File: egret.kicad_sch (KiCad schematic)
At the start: 36 parts, among them J6 ADB, Q1 MMBT3904, U10 EGRET, U12 LS1126, Y1 S3238E

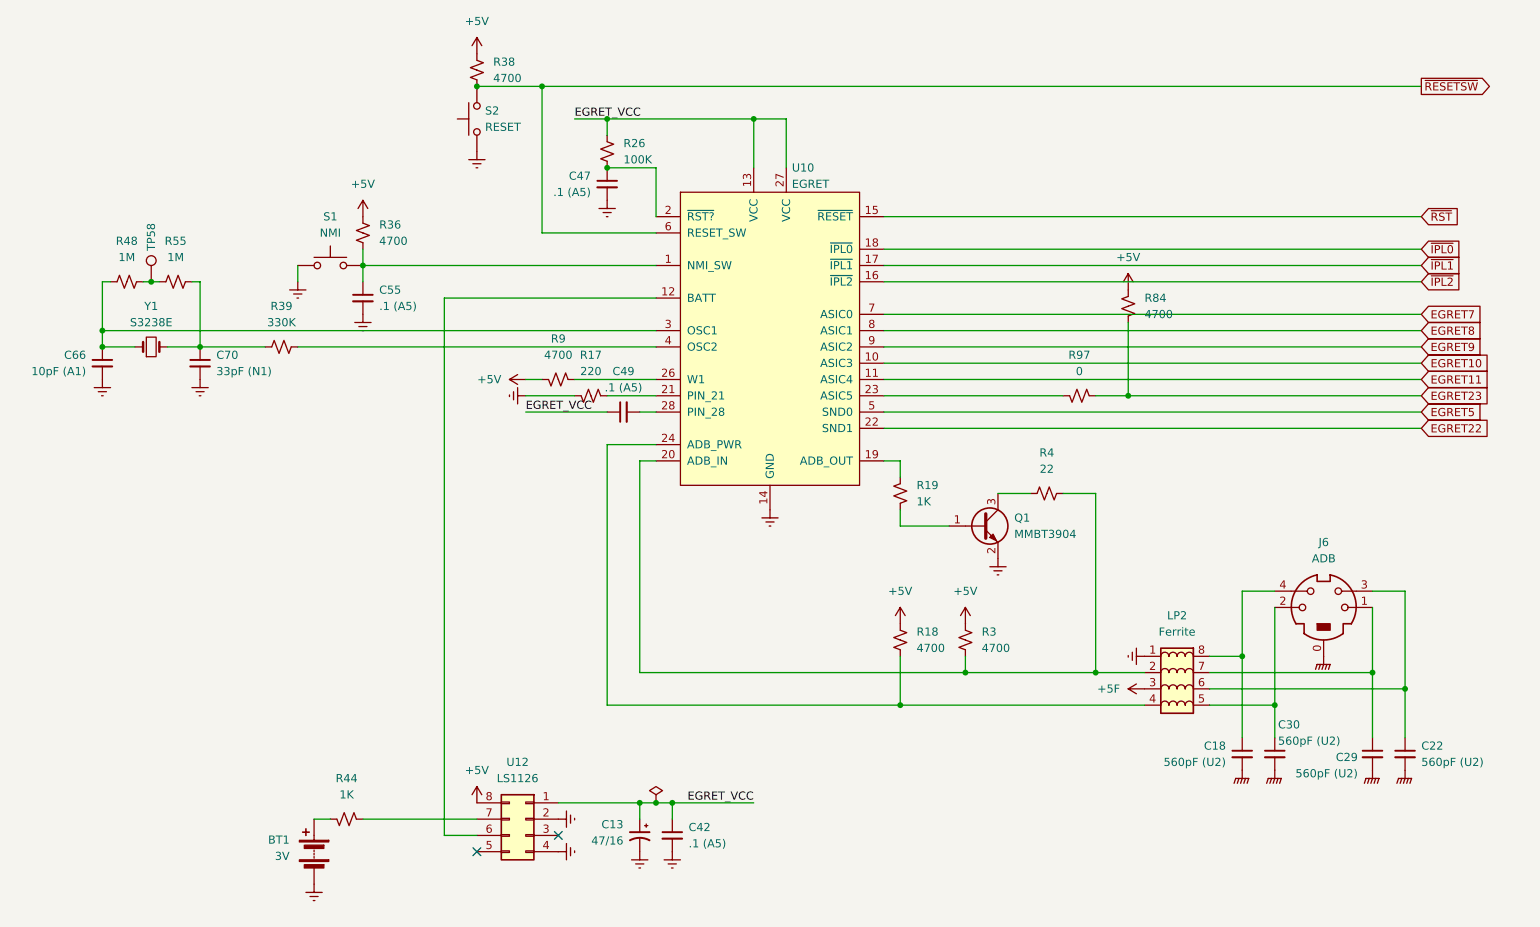
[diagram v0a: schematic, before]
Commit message: More schematic cleanup
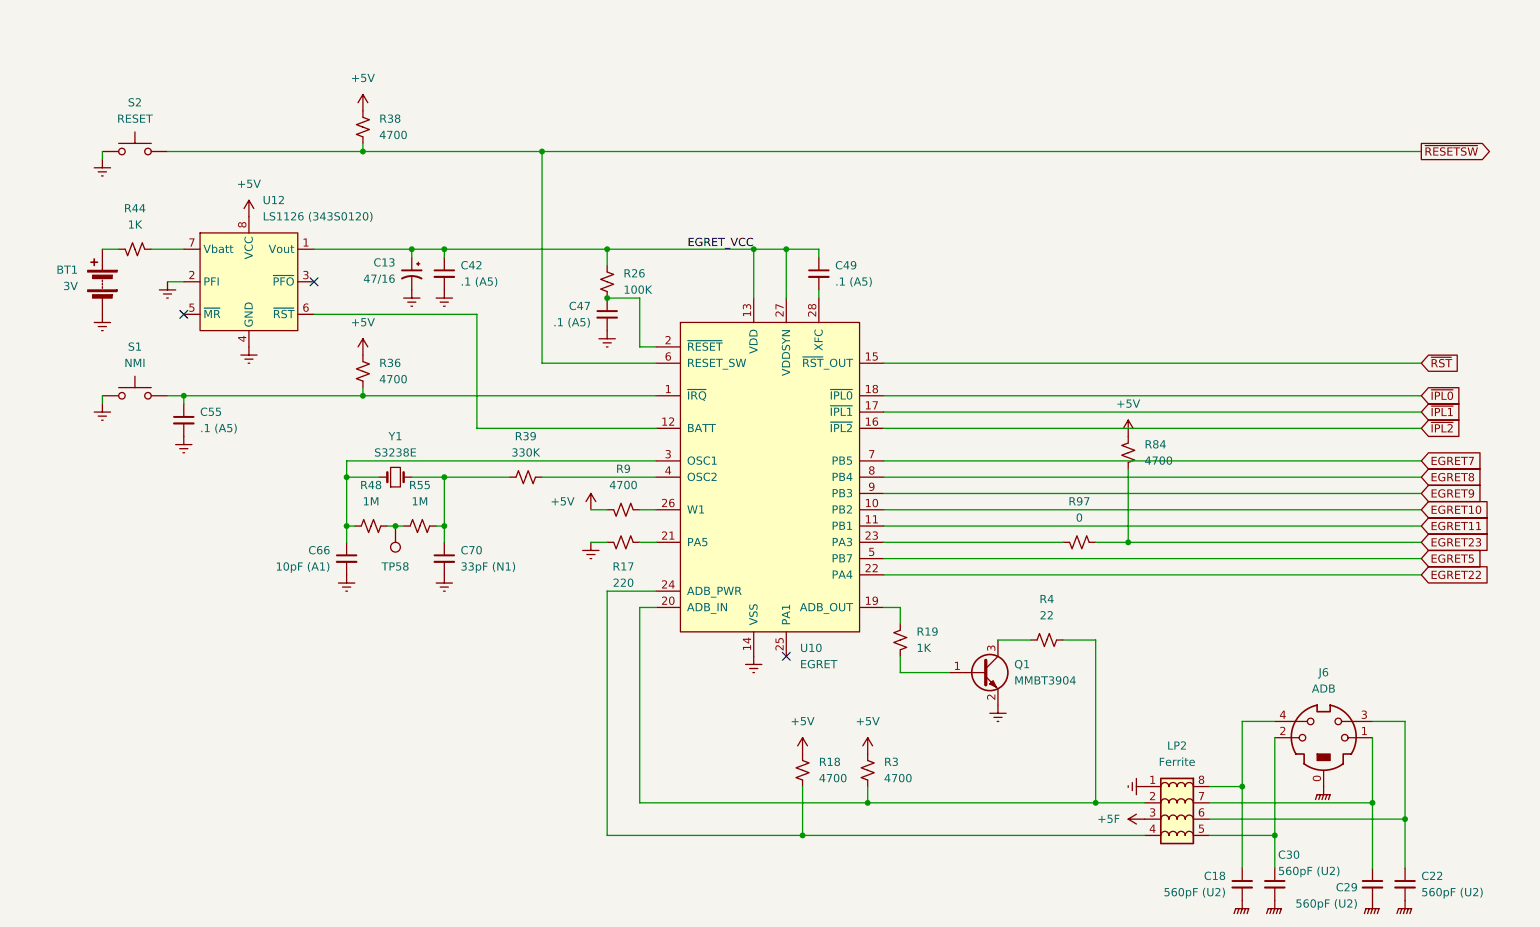
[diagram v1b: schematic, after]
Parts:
- U10: symbol AppleASIC:EGRET -> AppleASIC:EGRET_341S0851
- U12: value LS1126 -> LS1126 (343S0120); symbol Connector_Generic:Conn_02x04_Counter_Clockwise -> AppleASIC:LS1126_343S0120
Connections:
- no-connect marks 2 -> 3
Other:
- moved on the sheet: BT1, C13, C18, C22, C29, C30, C42, C47, C49, C55, C66, C70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
